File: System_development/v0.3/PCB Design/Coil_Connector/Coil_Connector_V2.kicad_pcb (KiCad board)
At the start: 2 copper layers, 15.5 x 26.7 mm, 4 parts, among them J1 Conn_Coaxial

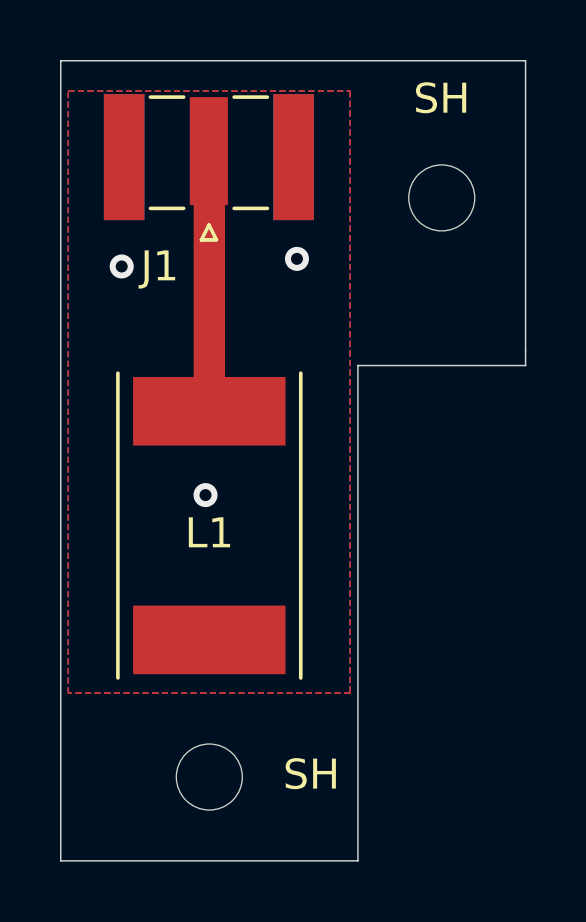
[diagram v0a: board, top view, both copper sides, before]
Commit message: Random
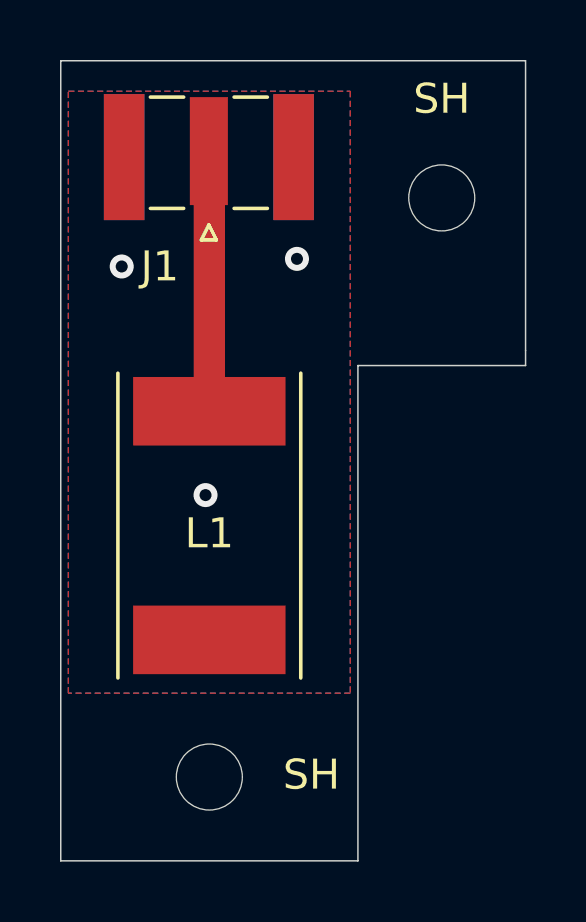
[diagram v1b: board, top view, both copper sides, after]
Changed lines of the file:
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@@
-    )
-  )
-  (zone (net 1) (net_name "GND") (layers F&B.Cu) (hatch edge 0.508)
-    (connect_pads (clearance 0.508))
-    (min_thickness 0.254) (filled_areas_thickness no)
-    (fill yes (thermal_gap 0.508) (thermal_bridge_width 0.508))
-    (polygon
-      (pts
-        (xy 143.764 117.856)
-        (xy 134.366 117.856)
-        (xy 134.366 97.79)
-        (xy 143.764 97.79)
-      )
     )
   )
